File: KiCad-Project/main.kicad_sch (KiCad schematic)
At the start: 35 parts, among them J1 USB_C_Receptacle_USB2.0, J2 BAT, J3 JTAG_TC2030, J4 RST, U1 nRF52840_moko_mk08, U2 SRV05-4, U3 MAX17048, U4 BQ24075RGT

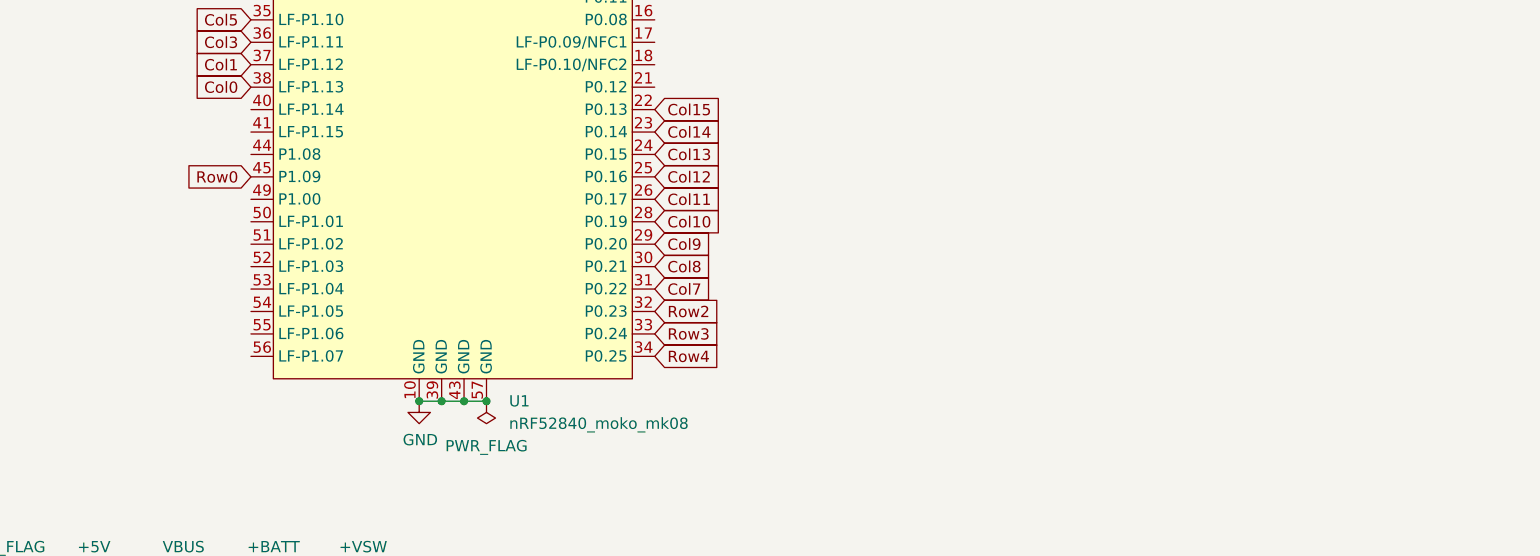
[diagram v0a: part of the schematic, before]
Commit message: Finish routing PCB
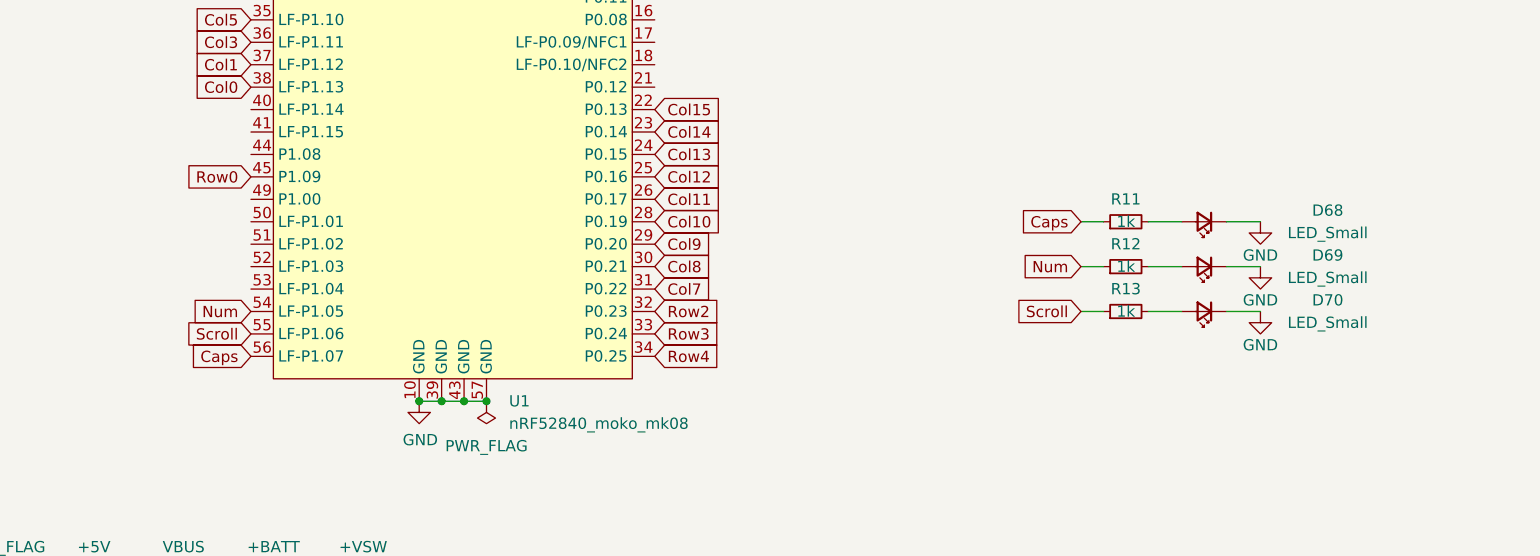
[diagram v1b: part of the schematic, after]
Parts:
- added D68, D69, D70: LED_Small, LED_THT:LED_D3.0mm, symbol Device:LED_Small
- added R11, R12, R13: 1k, Resistor_SMD:R_0402_1005Metric, symbol Device:R_Small
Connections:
- net GND: now also D68.1 (K), D69.1 (K), D70.1 (K)
- net Num: now reaches U1.54 (LF-P1.05)
- net Num: now also R12.1
- net Scroll: now reaches U1.55 (LF-P1.06)
- net Scroll: now also R13.1
- net Caps: now reaches U1.56 (LF-P1.07)
- net Caps: now also R11.1
- new net: D69.2 (A), R12.2
- new net: D68.2 (A), R11.2
- new net: D70.2 (A), R13.2
